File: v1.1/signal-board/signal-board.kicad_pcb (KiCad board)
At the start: 4 copper layers, 71 x 42 mm, 47 parts, among them IC1 74HCT245, J1 Jack-DC, J2 Conn_01x12, J3 JST SM, J4 Conn_01x16, J5 switch_jumpers, J6 switch_jumpers, SW1 SW_MEC_5G, SW2 SW_MEC_5G, U1 TPS63060, U2 ESP32-DEVKITC-32D

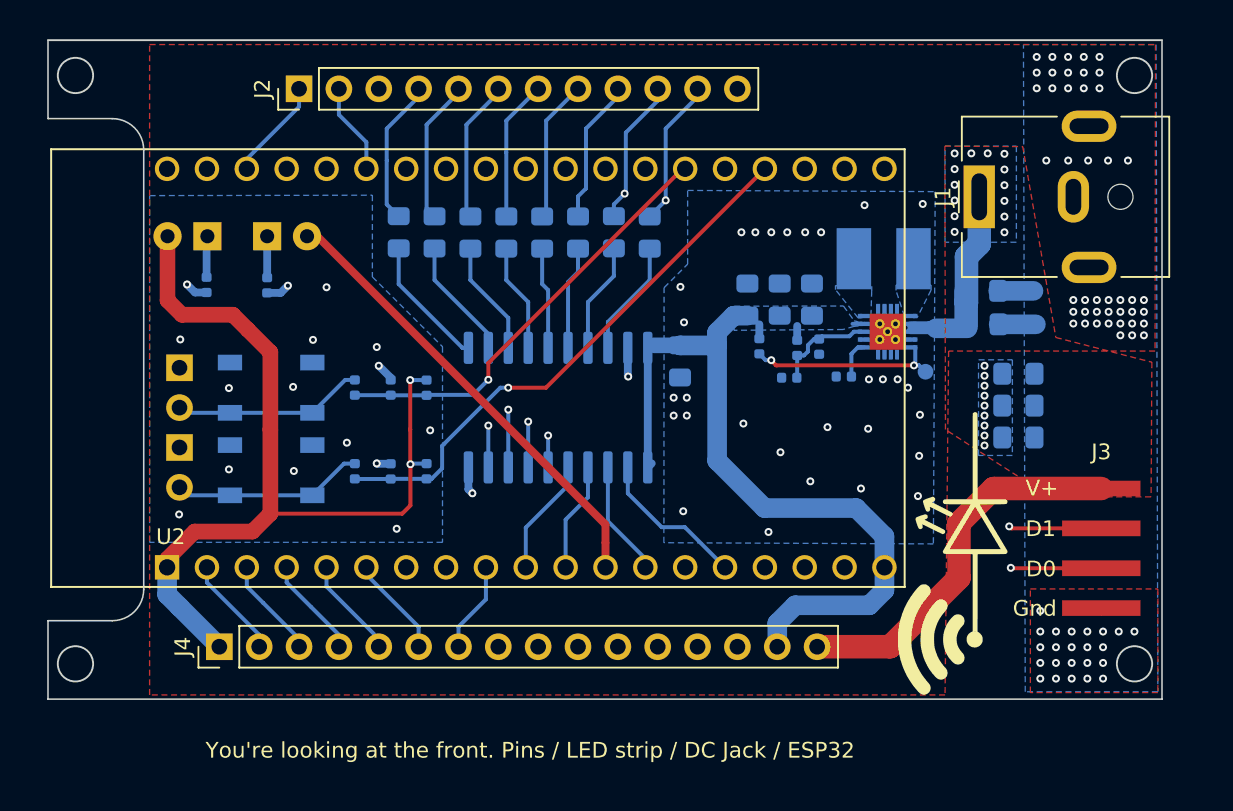
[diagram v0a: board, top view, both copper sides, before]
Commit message: circuit updates
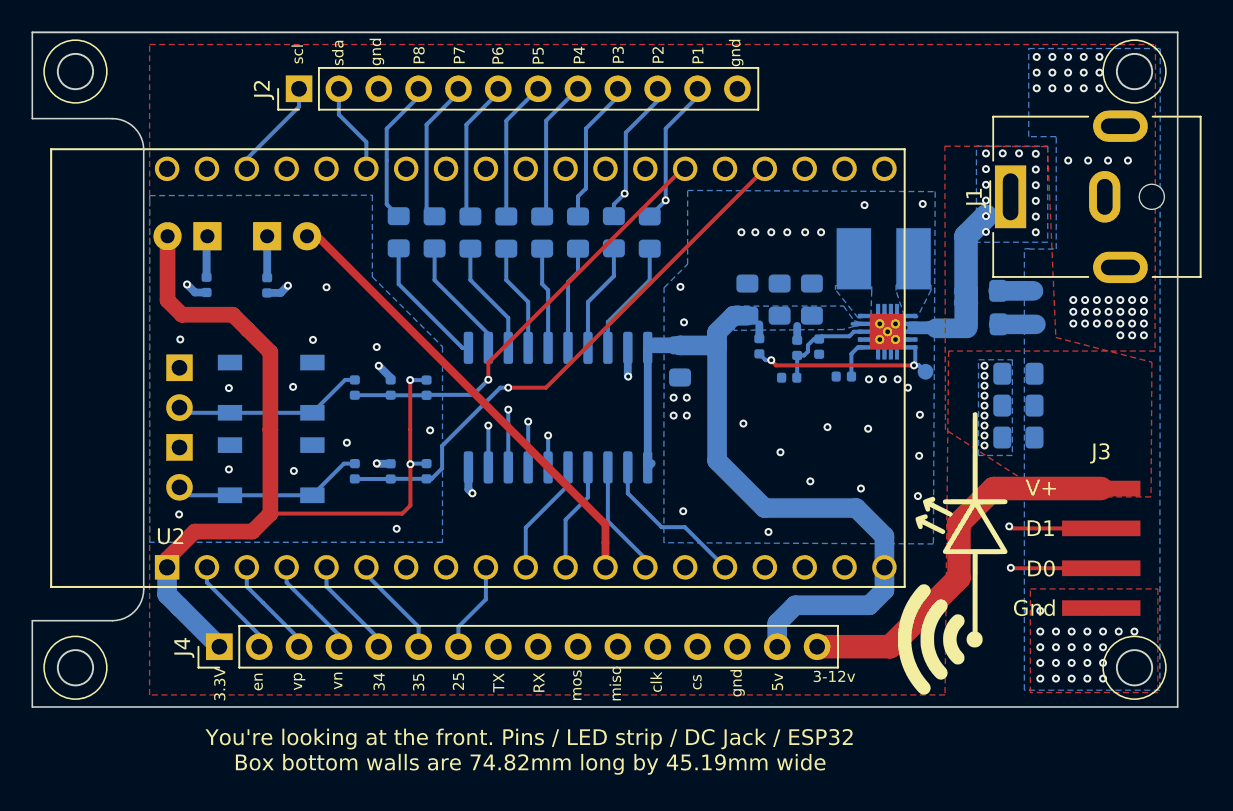
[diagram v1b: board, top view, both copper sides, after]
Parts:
- moved J1 2.00 mm to (159.7, 108.5)
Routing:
- net /3-12v: track 38.8 -> 37.0 mm
- net GND: vias 114 -> 113
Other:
- board size 71 x 42 mm -> 73 x 43 mm
- board text added: "25"
- board text added: "3-12v"
- board text added: "3.3V"
- board text added: "34"
- board text added: "35"
- board text added: "5v"
- board text added: "P1"
- board text added: "P2"
- board text added: "P3"
- board text added: "P4"
- board text added: "P5"
- board text added: "P6"
- board text added: "P7"
- board text added: "P8"
- board text added: "RX"
- board text added: "TX"
- board text added: "You're looking at the front. Pins / LED strip / DC Jack / ESP32 Box bottom walls are 74.82mm long by 45.19mm wide"
- board text added: "clk"
- board text added: "cs"
- board text added: "en"
- board text added: "gnd"
- board text added: "miso"
- board text added: "mosi"
- board text added: "scl"
- board text added: "sda"
- board text added: "vn"
- board text added: "vp"
- board text removed: "You're looking at the front. Pins / LED strip / DC Jack / ESP32"
